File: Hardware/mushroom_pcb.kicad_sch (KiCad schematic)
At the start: 54 parts, among them J1 Conn_01x04, J10 Screw_Terminal_01x03, J2 Conn_01x07_Pin, J3 Screw_Terminal_01x02, J5 Screw_Terminal_01x02, J6 Screw_Terminal_01x02, J7 Conn_01x03_Pin, J8 Conn_01x04_Pin, J9 Barrel_Jack, Q3 AO3400A, Q4 AO3400A, SW1 SW_Push, SW2 SW_Push, SW3 RotaryEncoder_Switch, U1 ESP32-WROOM-32E, U2 LM2596S-5, U3 ME6211C33M5, U4 PC817

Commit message: cambios menores, conectores + octo
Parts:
- J9: footprint Connector_BarrelJack:BarrelJack_SwitchcraftConxall_RAPC10U_Horizontal -> Connector_BarrelJack:BarrelJack_CUI_PJ-102AH_Horizontal
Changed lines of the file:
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@@
 			)
 		)
-		(property "Footprint" "Connector_BarrelJack:BarrelJack_SwitchcraftConxall_RAPC10U_Horizontal"
+		(property "Footprint" "Connector_BarrelJack:BarrelJack_CUI_PJ-102AH_Horizontal"
 			(at 130.81 61.976 0)
 			(hide yes)

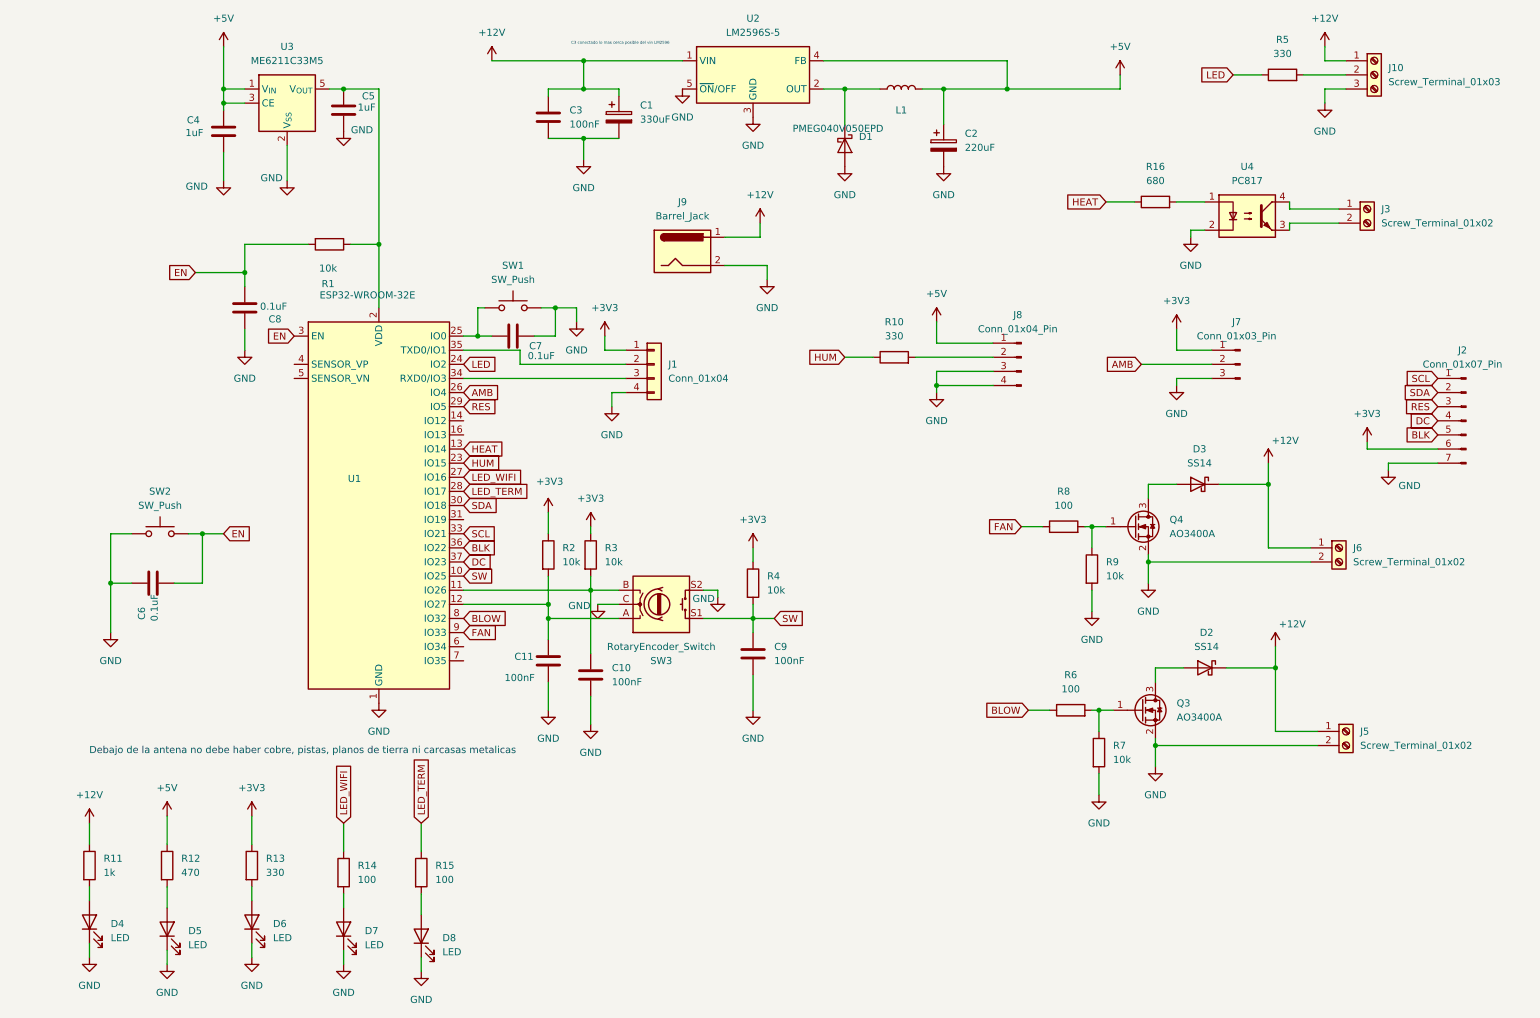
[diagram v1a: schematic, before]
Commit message: Cambios en arch de fabricacion
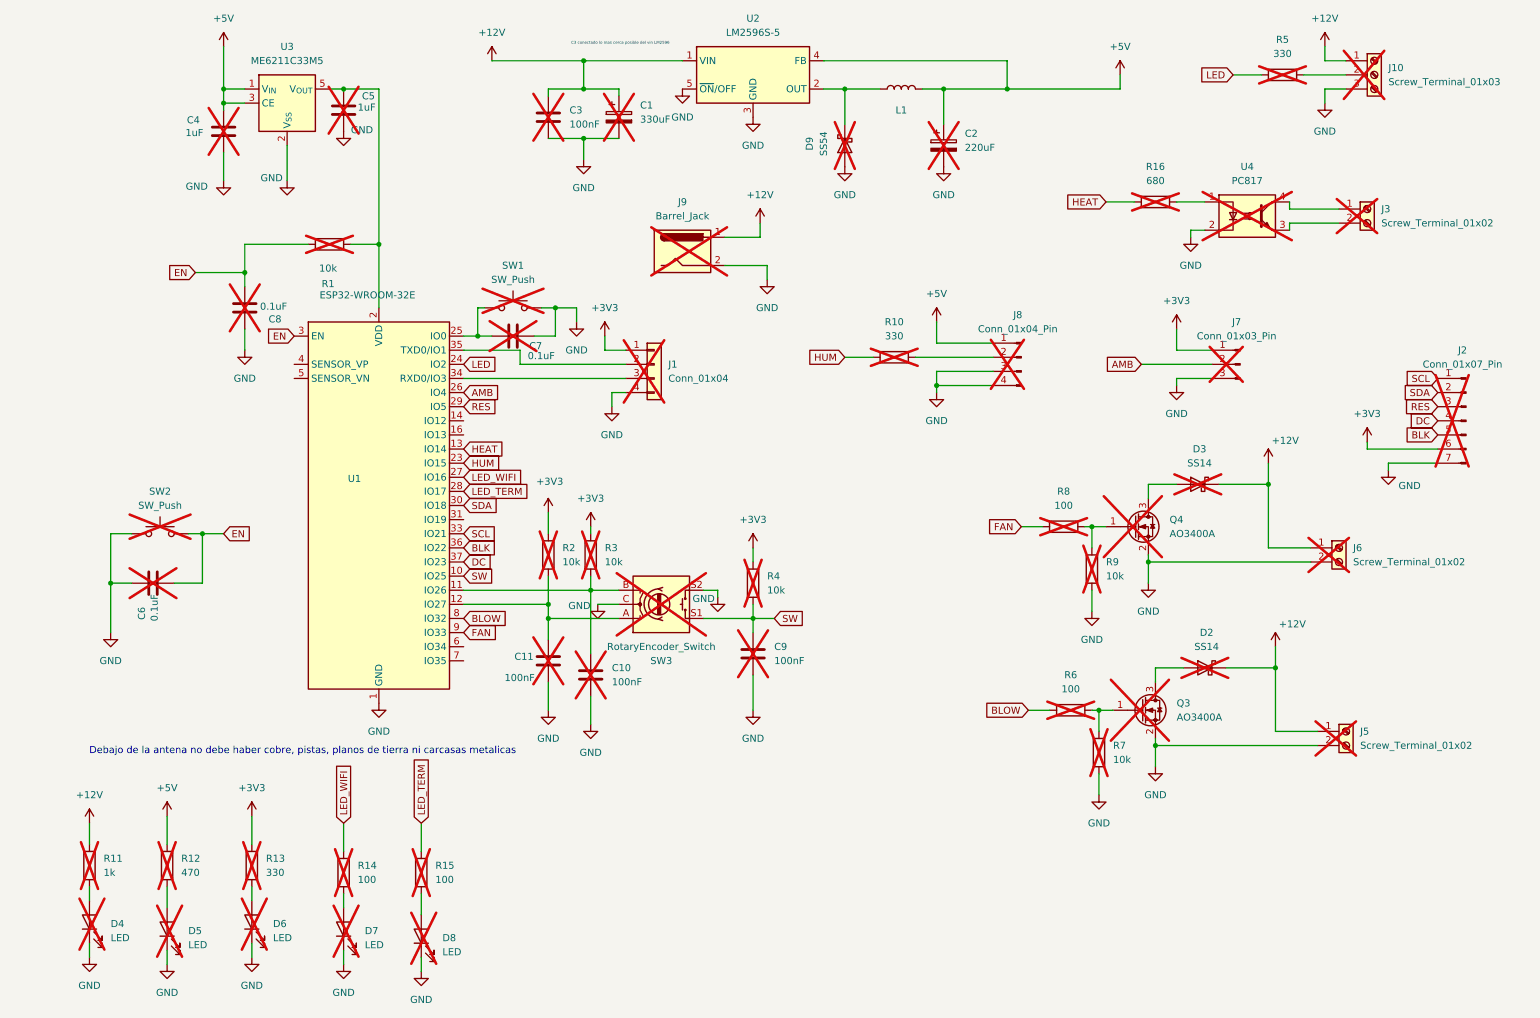
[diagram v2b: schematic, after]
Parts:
- removed D1: PMEG040V050EPD, Package_TO_SOT_SMD:Nexperia_CFP15_SOT-1289, symbol Diode:PMEG040V050EPD
- added D9: SS54, Diode_SMD:D_SMA, symbol Diode:SS14
- C1, C10, C11, C2, C3, C4, C5, C6, C7, C8, C9, D2, D3, D4, D5, D6, D7, D8, J1, J10, J2, J3, J5, J6, J7, J8, J9, Q3, Q4, R1, R10, R11, R12, R13, R14, R15, R16, R2, R3, R4, R5, R6, R7, R8, R9, SW1, SW2, SW3, U4: now not fitted
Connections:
- net GND: now also D9.2 (A)
- net at L1.1, U2.2 (OUT): now also D9.1 (K)
